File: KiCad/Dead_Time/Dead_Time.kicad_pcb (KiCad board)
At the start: 2 copper layers, 61.5 x 39.2 mm, 13 parts, among them Q7 PNP_BC558, U1 74AUC2G04, U2 MCP6002

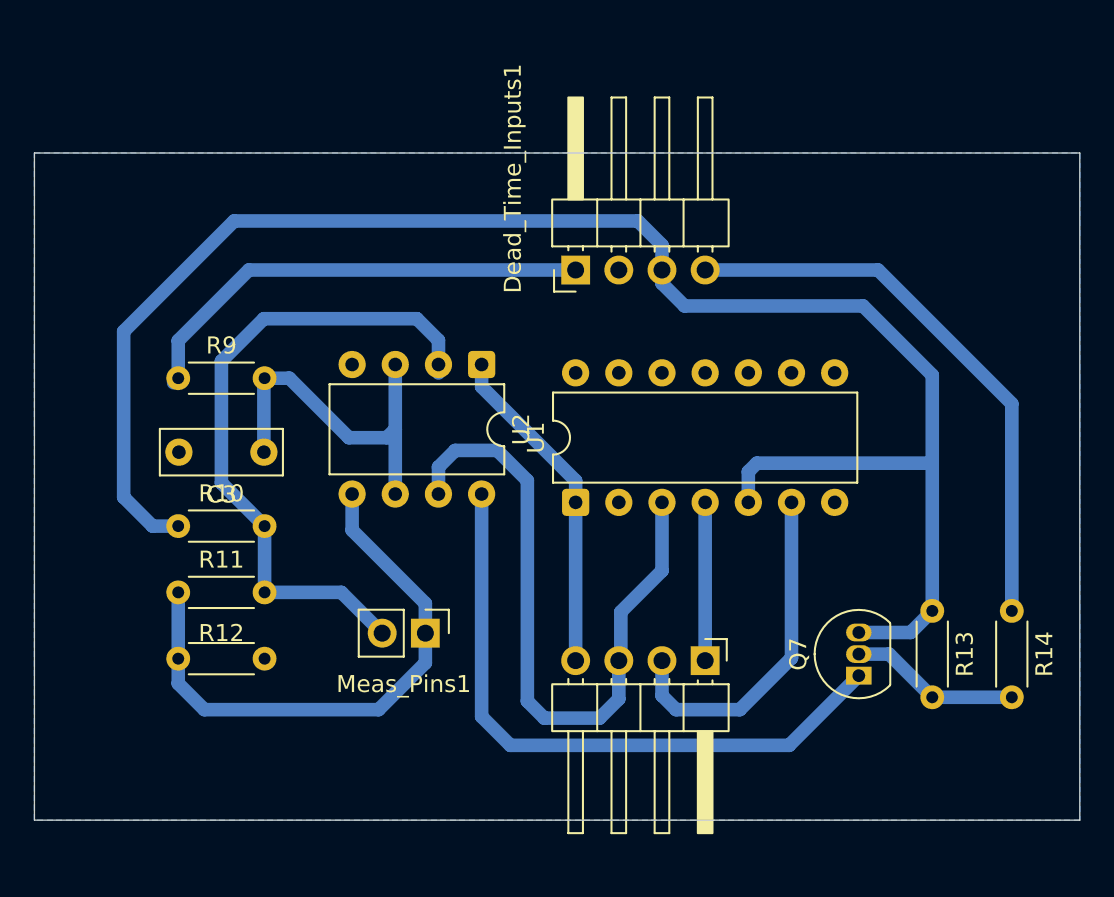
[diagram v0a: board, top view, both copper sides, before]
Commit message: pcb layouts done
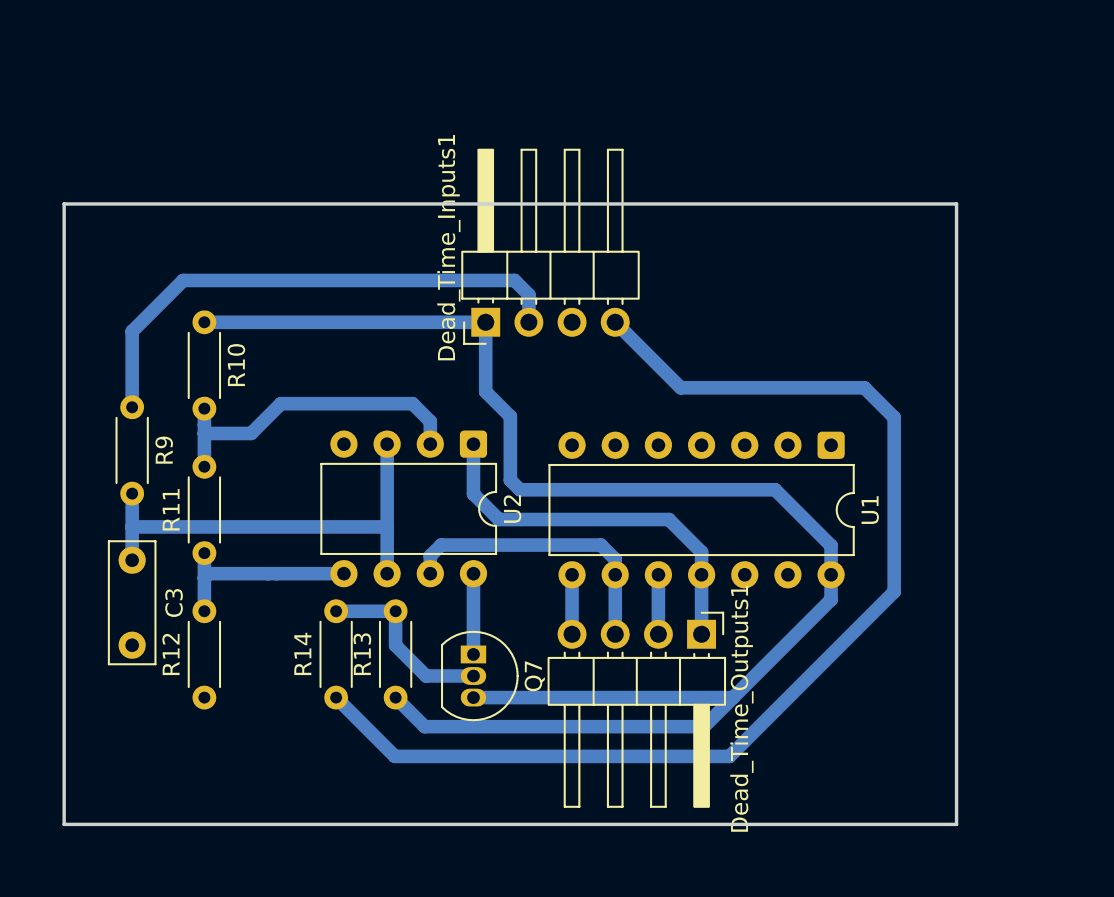
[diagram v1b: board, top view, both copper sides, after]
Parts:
- removed Meas_Pins1: Conn_01x02_Pin, Connector_PinHeader_2.54mm:PinHeader_1x02_P2.54mm_Vertical
- moved R14 40.1 mm to (94.8, 124.8), turned to 90 degrees
- moved R13 32.0 mm to (98.2, 124.8), turned to 90 degrees
- moved Q7 22.7 mm to (102.8, 122.2), turned to -90 degrees
- moved U1 15.4 mm to (123.9, 109.9), turned to -90 degrees
- moved R10 12.1 mm to (87.0, 102.7), turned to -90 degrees
- moved C3 10.0 mm to (82.8, 116.7), turned to -90 degrees
- moved Dead_Time_Inputs1 6.12 mm to (103.5, 102.7)
- moved U2 4.71 mm to (102.8, 109.9)
- moved R12 4.22 mm to (87.0, 124.8), turned to 90 degrees
- moved R9 3.20 mm to (82.8, 107.7), turned to -90 degrees
- moved R11 2.78 mm to (87.0, 116.3), turned to 90 degrees
- moved Dead_Time_Outputs1 1.56 mm to (116.2, 121.1)
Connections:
- Dead_Time_Inputs1 pad 1: /PWM_In -> +5V
- Dead_Time_Inputs1 pad 2: GND -> /PWM_In
- Dead_Time_Inputs1 pad 3: +5V -> GND
- Dead_Time_Outputs1 pad 1: /PWM2_NOT -> /PWM1
- Dead_Time_Outputs1 pad 4: /PWM1 -> /PWM2_NOT
- U1 pad 1: /PWM1 -> (no net)
- U1 pad 10: (no net) -> /PWM1_NOT
- U1 pad 11: (no net) -> /PWM1
- U1 pad 14: (no net) -> +5V
- U1 pad 2: GND -> (no net)
- U1 pad 3: /PWM2 -> (no net)
- U1 pad 4: /PWM2_NOT -> (no net)
- U1 pad 5: +5V -> (no net)
- U1 pad 6: /PWM1_NOT -> (no net)
- U1 pad 7: (no net) -> GND
- U1 pad 8: (no net) -> /PWM2_NOT
- U1 pad 9: (no net) -> /PWM2
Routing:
- net /on/off: track 33.5 -> 67.3 mm
- net /KILL_SWITCH: track 37.7 -> 4.75 mm
- net /PWM2: track 39.8 -> 16.9 mm
- net /Meas_VStep2: track 33.4 -> 11.7 mm
- net /Meas_VStep1: track 38.8 -> 19.2 mm
- net /PWM1_NOT: track 20.4 -> 3.50 mm
- net /PWM2_NOT: track 9.31 -> 3.50 mm
- net +5V: track 100.5 -> 94.9 mm
- net Net-(U2A-+): track 20.8 -> 26.0 mm
- net /PWM_In: track 27.0 -> 31.0 mm
- net /PWM1: track 19.4 -> 22.6 mm
- net Net-(Q7-B): track 10.1 -> 10.8 mm
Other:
- board size 61.5 x 39.2 mm -> 52.5 x 36.5 mm
